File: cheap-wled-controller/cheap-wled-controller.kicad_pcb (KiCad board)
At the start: 2 copper layers, 100 x 50 mm, 47 parts, among them J10 Conn_01x05_Pin, J2 USB_C_Receptacle, J4 Conn_02x05_Odd_Even, J6 Conn_01x05_Pin, J7 Conn_01x02_Pin, J8 Conn_01x07_Pin, Q3 NMOS, SW1 SW_Push, U1 USBLC6-2SC6, U3 CH224K, U4 MX5014S, U5 ESP32-S3-WROOM-1-N4R2, U7 TPS54202DDC, U9 AMS1117-3.3

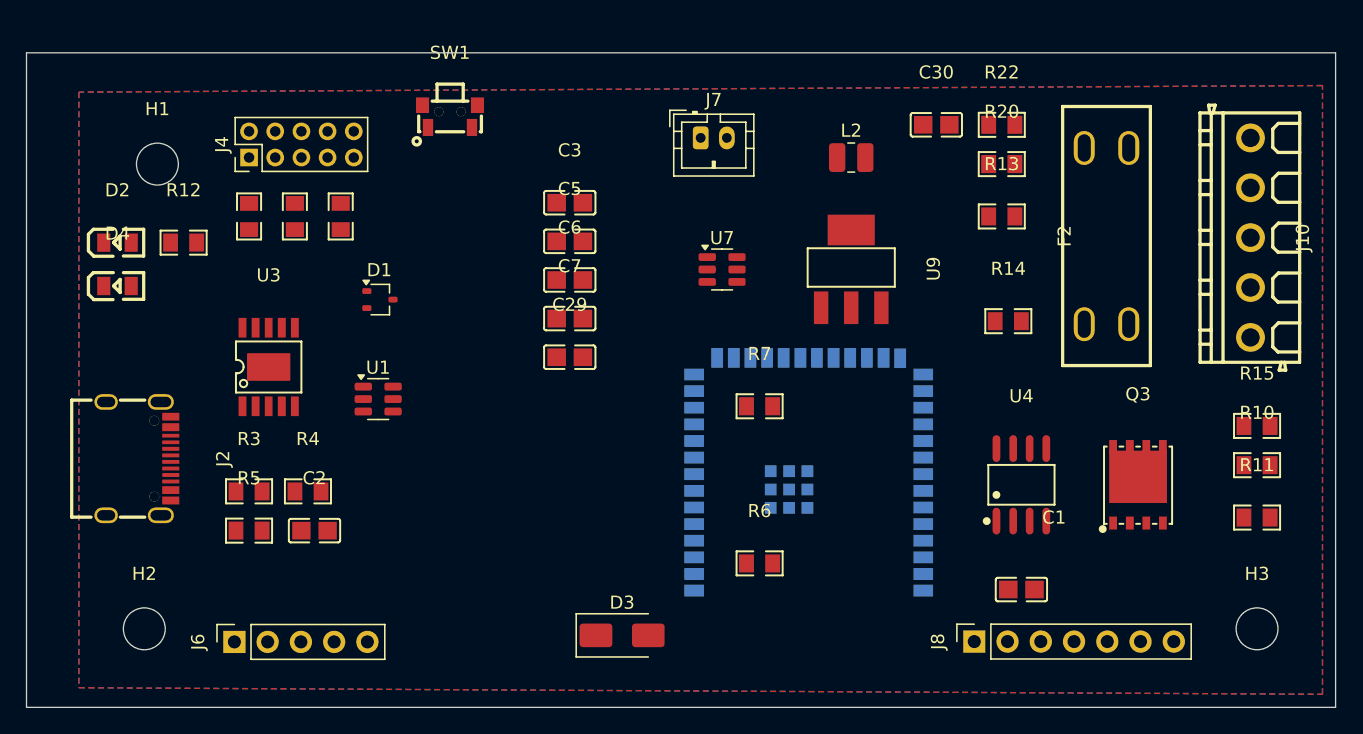
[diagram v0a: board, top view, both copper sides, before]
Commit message: some traces
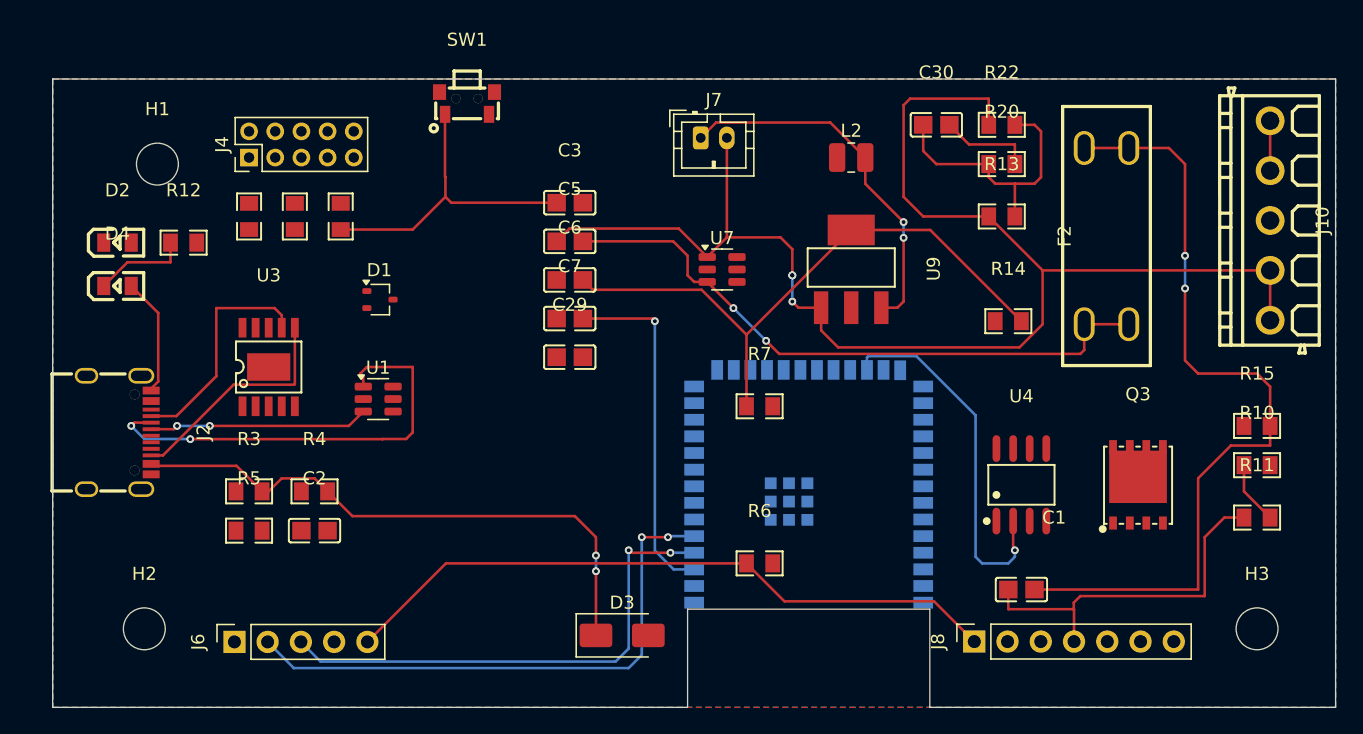
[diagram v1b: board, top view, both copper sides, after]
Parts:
- moved J2 2.50 mm to (17.1, 39.0)
- moved J10 1.99 mm to (105.0, 22.8)
- moved SW1 1.64 mm to (43.6, 13.8)
- moved U5 0.92 mm to (69.8, 43.1)
- moved R4 0.50 mm to (32.0, 43.5)
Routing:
- net GND: track 0.00 -> 168.9 mm, vias 0 -> 3
- net +3.3V: track 0.00 -> 98.2 mm
- net /VBUS_C: track 0.00 -> 92.8 mm, vias 0 -> 4
- net /V_LED: track 0.00 -> 62.6 mm, vias 0 -> 2
- net /GPIO5: track 0.00 -> 42.9 mm, vias 0 -> 2
- net /GPIO4: track 0.00 -> 38.7 mm, vias 0 -> 2
- net +5V: track 0.00 -> 35.4 mm, vias 0 -> 2
- net /D-: track 0.00 -> 34.1 mm, vias 0 -> 2
- net /MOS_1: track 0.00 -> 28.2 mm, vias 0 -> 1
- net Net-(U5-EN): track 0.00 -> 26.7 mm, vias 0 -> 1
- net /FB: track 0.00 -> 21.0 mm
- net Net-(D1-K2): track 0.00 -> 17.6 mm
- net Net-(D1-K1): track 0.00 -> 17.5 mm
- net /D+: track 0.00 -> 16.8 mm, vias 0 -> 2
- net Net-(D4-A): track 0.00 -> 7.35 mm
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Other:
- board size 100 x 50 mm -> 98 x 48 mm
